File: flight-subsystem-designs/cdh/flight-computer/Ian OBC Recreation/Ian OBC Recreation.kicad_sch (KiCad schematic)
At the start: 44 parts, among them J1 Conn_01x03, J2 Conn_01x03, J3 Conn_01x03, J4 Conn_01x03, J5 Conn_01x03, J6 Conn_01x03, J8 Conn_02x26_Odd_Even, Q1 AON6411, U1 BEAGLEBONEBLACK, U2 TPS2400DBVR, U3 TCAN337G, U4 MCP7940N-xSN, U5 ADM3485EARZ, U6 MAX706RESA+T, U7 TMP36xS

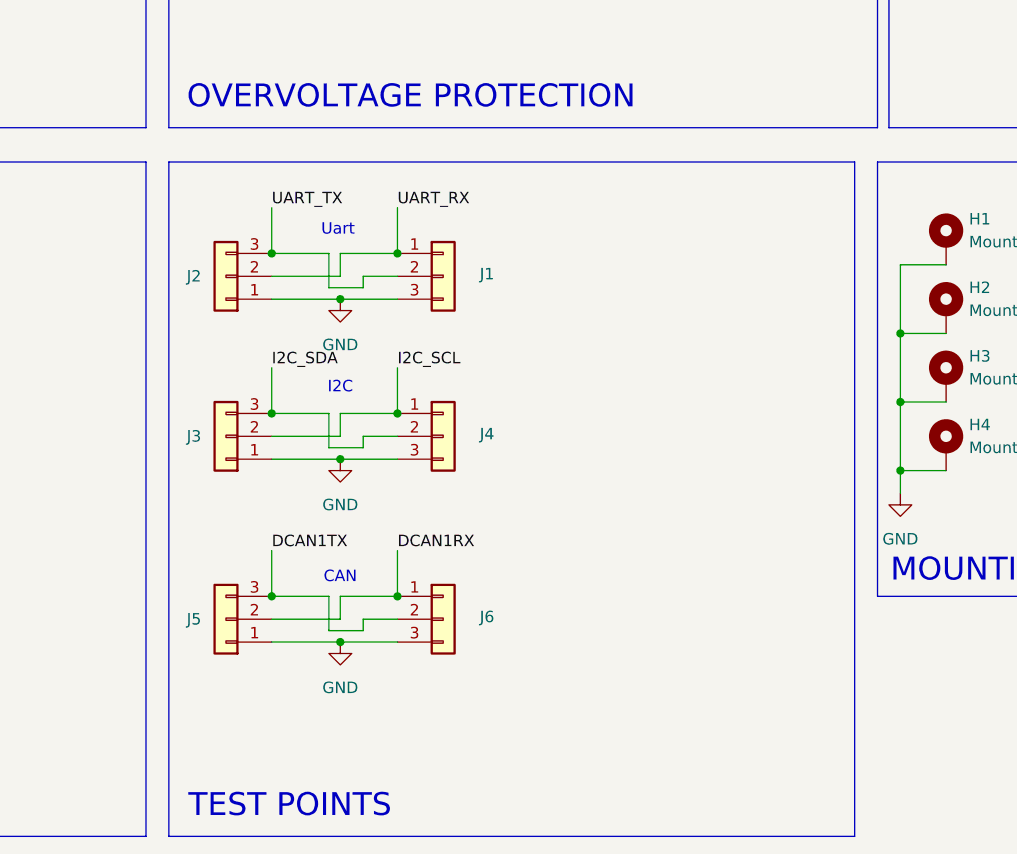
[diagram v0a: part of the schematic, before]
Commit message: Routing is fixed unless I missed something
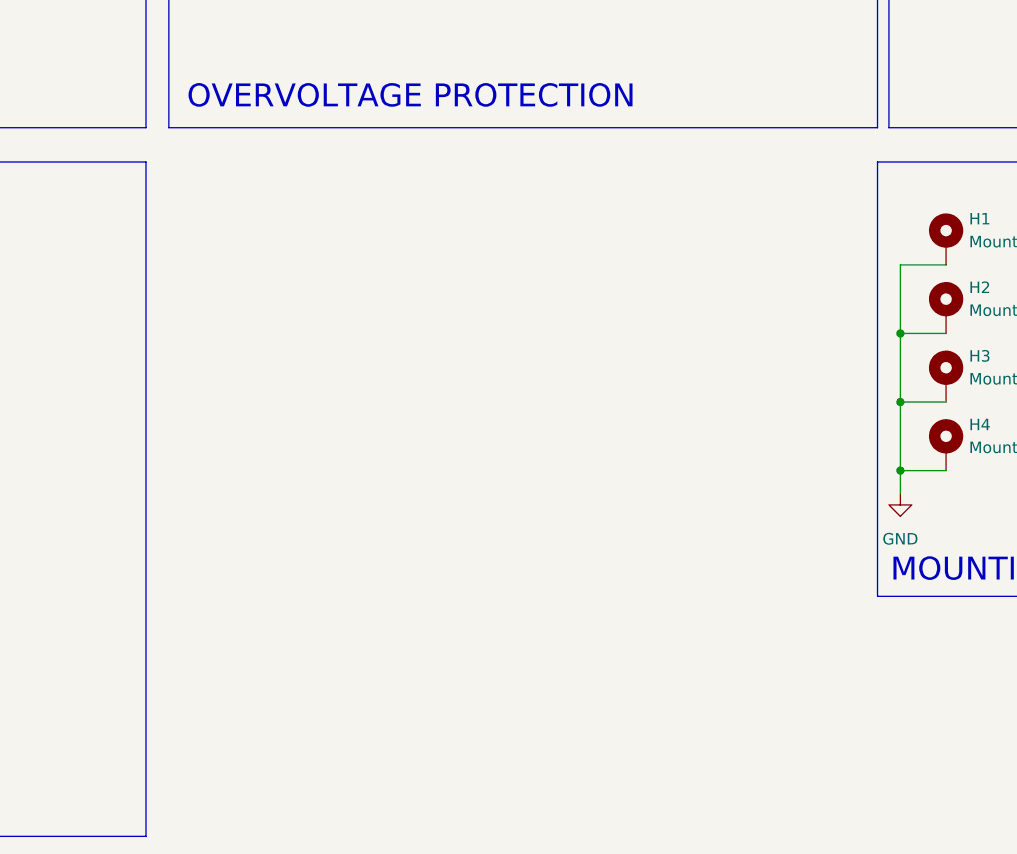
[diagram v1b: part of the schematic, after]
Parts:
- removed J1, J2, J3, J4, J5, J6: Conn_01x03, Connector_PinHeader_2.54mm:PinHeader_1x03_P2.54mm_Vertical, symbol Connector_Generic:Conn_01x03
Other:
- note removed: "CAN"
- note removed: "I2C"
- note removed: "TEST POINTS"
- note removed: "Uart"

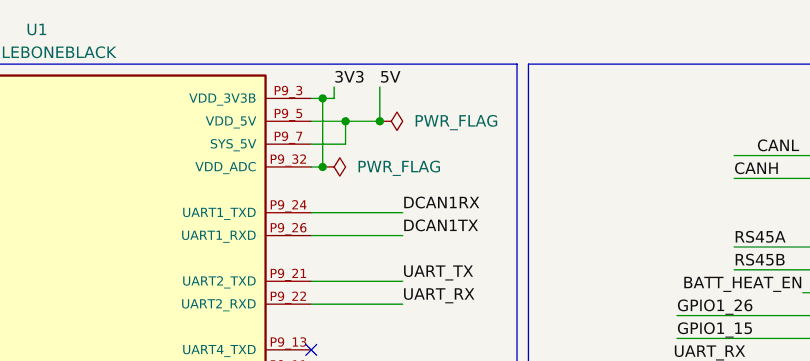
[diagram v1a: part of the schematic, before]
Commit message: Intermediate fixes, still WIP
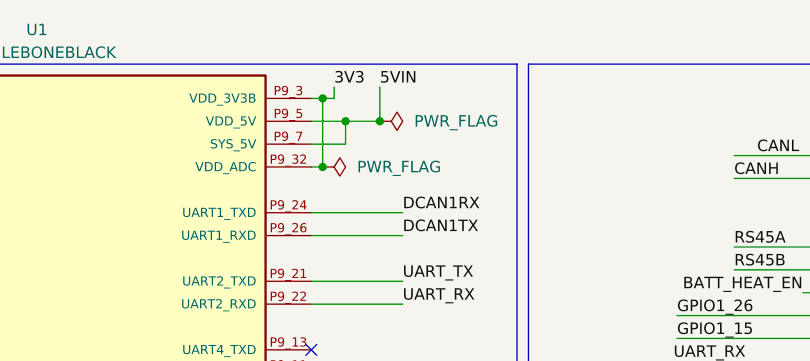
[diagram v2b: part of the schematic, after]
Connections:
- net 5VIN is gone; now on net SYS_5V: J8.77 (Pin_25), J8.78 (Pin_26)
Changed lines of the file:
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@@
 		)
 	)
-	(label "5V"
+	(label "5VIN"
 		(at 95.25 16.51 0)
 		(effects
